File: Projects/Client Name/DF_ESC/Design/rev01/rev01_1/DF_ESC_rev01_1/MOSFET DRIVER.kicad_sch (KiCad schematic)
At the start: 1 part, among them U1 DRV8302DCAR

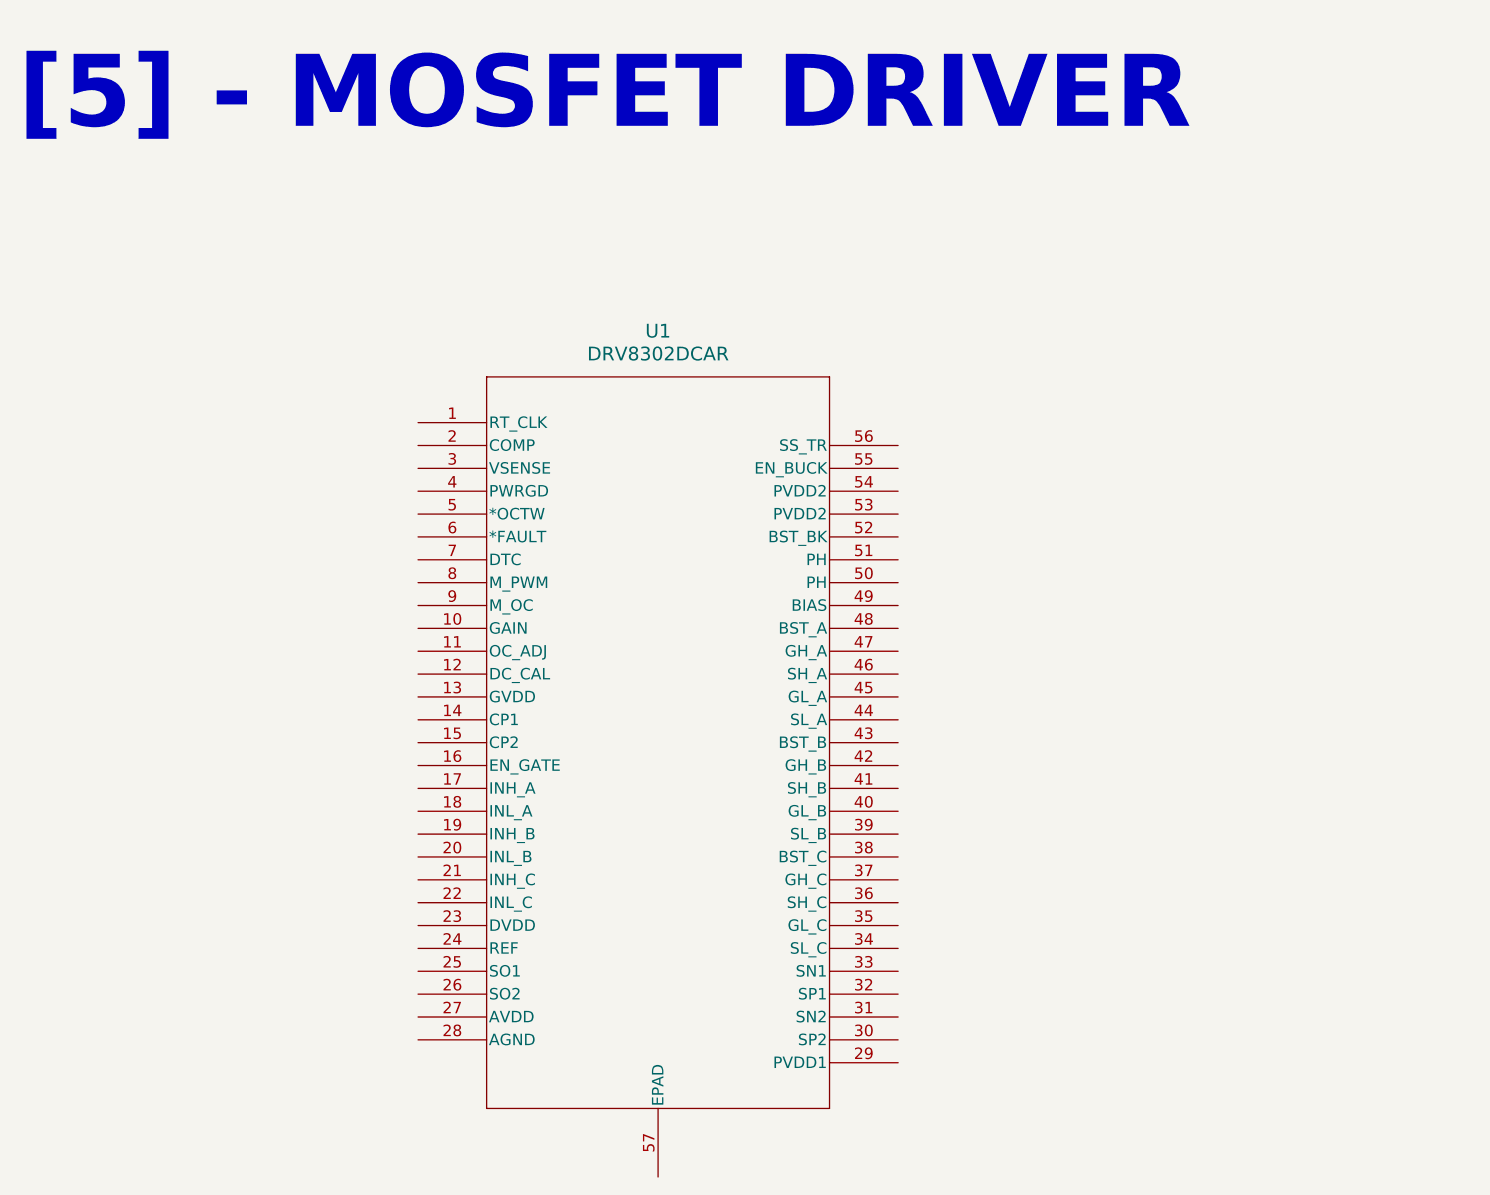
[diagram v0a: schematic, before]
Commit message: Udpate 23-01-2024_Prueba
Solo se borro para probar cambio de carpeta KICAD_directorio por Github
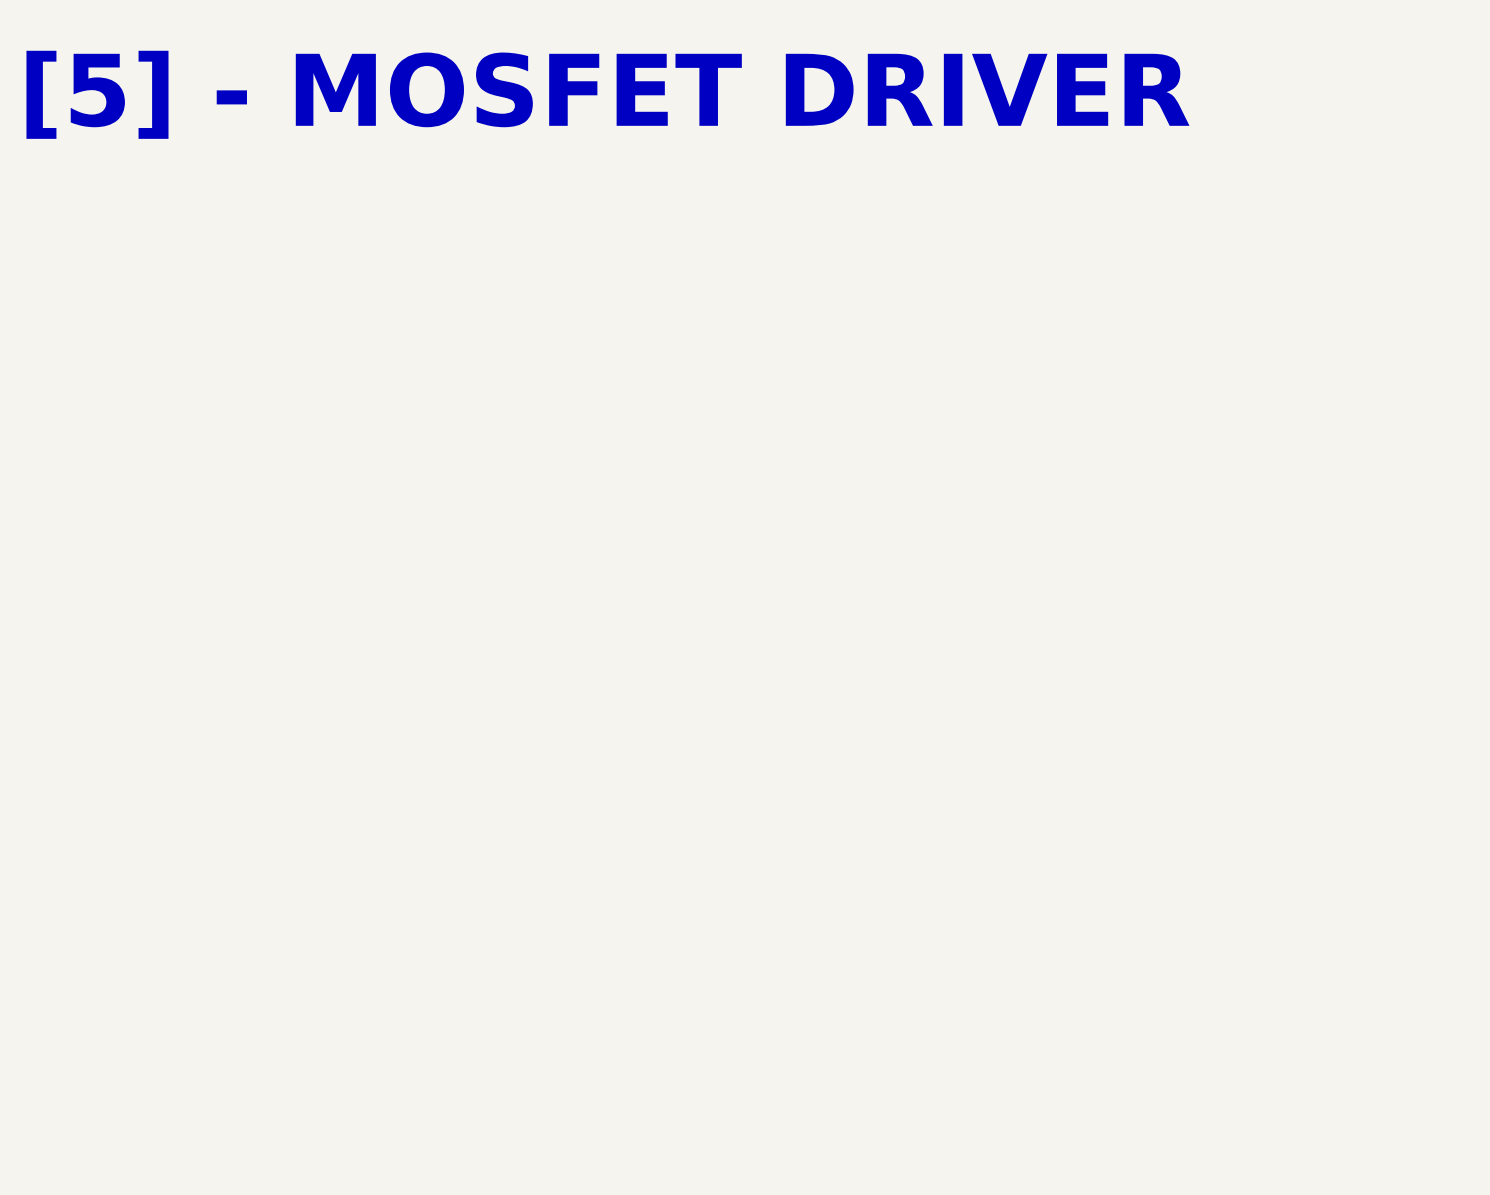
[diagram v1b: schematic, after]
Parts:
- removed U1: DRV8302DCAR, DCA56_6P35X3P61, symbol DRV8302:DRV8302DCAR
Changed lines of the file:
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@@
     (effects (font (size 8 8) bold) (justify left bottom))
   )
-  (symbol (lib_id "DRV8302:DRV8302DCAR") (at 129.54 59.69 0) (unit 1)
-    (in_bom yes) (on_board yes) (dnp no) (fields_autoplaced)
-    (property "Reference" "U1" (at 156.21 49.53 0)
-      (effects (font (size 1.524 1.524)))
-    )
-    (property "Value" "DRV8302DCAR" (at 156.21 52.07 0)
-      (effects (font (size 1.524 1.524)))
-    )
-    (property "Footprint" "DCA56_6P35X3P61" (at 157.48 53.34 0)
-      (effects (font (size 1.27 1.27) italic) hide)
-    )
-    (property "Datasheet" "DRV8302DCAR" (at 157.48 50.8 0)
-      (effects (font (size 1.27 1.27) italic) hide)
-    )
-    (pin "42")
-    (pin "12")
-    (pin "56")
-    (pin "14")
-    (pin "54")
-    (pin "34")
-    (pin "27")
-    (pin "36")
-    (pin "39")
-    (pin "28")
-    (pin "37")
-    (pin "55")
-    (pin "3")
-    (pin "7")
-    (pin "19")
-    (pin "38")
-    (pin "24")
-    (pin "43")
-    (pin "45")
-    (pin "5")
-    (pin "17")
-    (pin "2")
-    (pin "21")
-    (pin "47")
-    (pin "40")
-    (pin "30")
-    (pin "50")
-    (pin "51")
-    (pin "9")
-    (pin "23")
-    (pin "10")
-    (pin "13")
-    (pin "26")
-    (pin "35")
-    (pin "29")
-    (pin "33")
-    (pin "48")
-    (pin "49")
-    (pin "16")
-    (pin "1")
-    (pin "25")
-    (pin "41")
-    (pin "11")
-    (pin "52")
-    (pin "57")
-    (pin "53")
-    (pin "15")
-    (pin "44")
-    (pin "46")
-    (pin "4")
-    (pin "31")
-    (pin "22")
-    (pin "6")
-    (pin "8")
-    (pin "20")
-    (pin "32")
-    (pin "18")
-    (instances
-      (project "DF_ESC_rev01_1"
-        (path "/e63e39d7-6ac0-4ffd-8aa3-1841a4541b55/ebfeafe7-4d70-4ef9-bb18-a00f088a6e19"
-          (reference "U1") (unit 1)
-        )
-      )
-    )
-  )
 )
